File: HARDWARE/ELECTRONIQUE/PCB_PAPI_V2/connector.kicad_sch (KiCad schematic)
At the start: 20 parts, among them J1 USB4110-GF-A, J3 XT30PW-M, J5 SM12B-SRSS-TB_LF__SN_

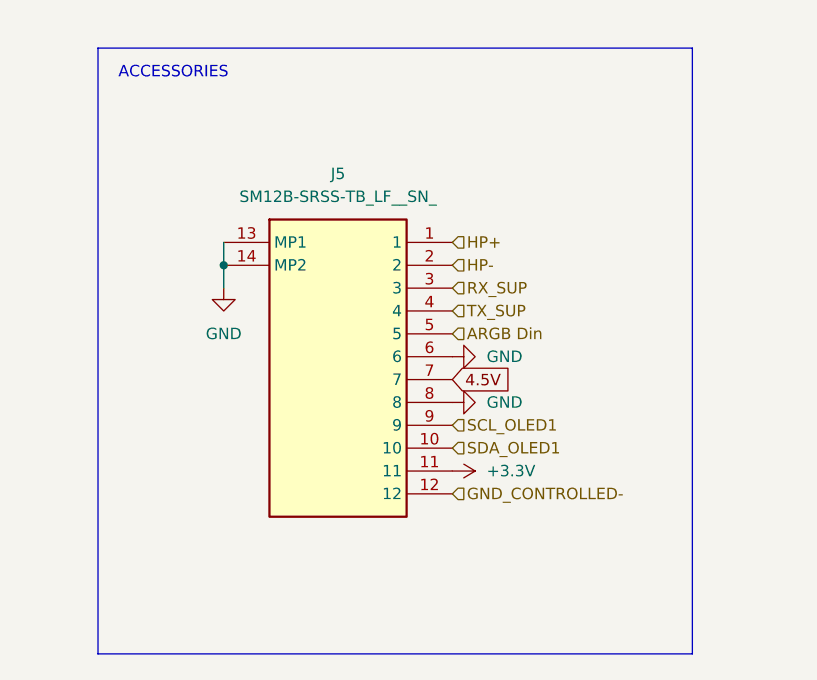
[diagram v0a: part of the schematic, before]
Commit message: up
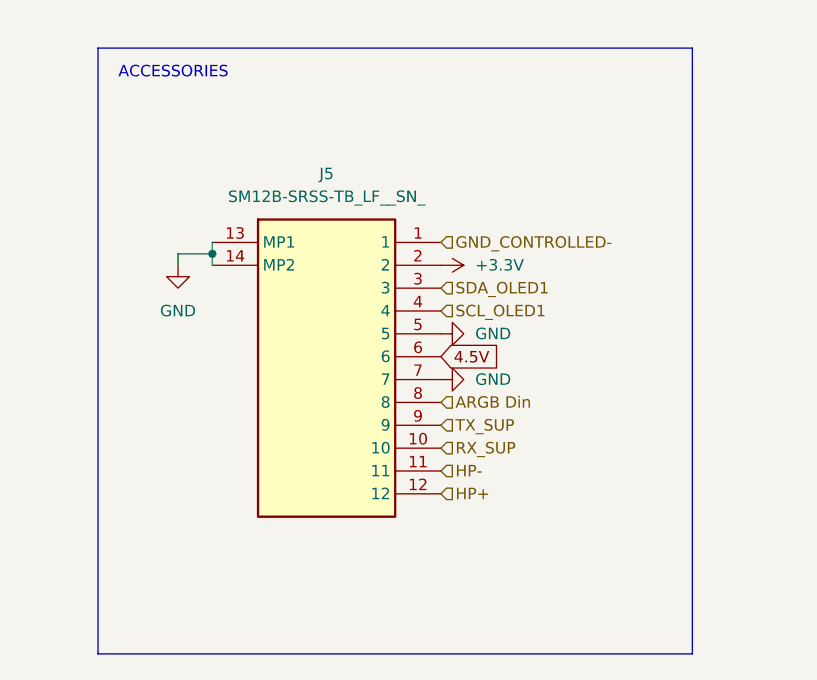
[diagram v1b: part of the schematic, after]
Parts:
- USBJUMP1: footprint Connector_PinHeader_1.00mm:PinHeader_2x04_P1.00mm_Vertical_SMD -> Connector_PinHeader_1.27mm:PinHeader_2x04_P1.27mm_Vertical_SMD
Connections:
- net +3.3V: now also J5.2; no longer J5.11
- net 4.5V: now also J5.6; no longer J5.7
- net ARGB Din: now also J5.8; no longer J5.5
- net GND: now also J5.5, J5.7; no longer J5.6, J5.8
- net GND_CONTROLLED-: now also J5.1; no longer J5.12
- net HP+: now also J5.12; no longer J5.1
- net HP-: now also J5.11; no longer J5.2
- net RX_SUP: now also J5.10; no longer J5.3
- net SCL_OLED1: now also J5.4; no longer J5.9
- net SDA_OLED1: now also J5.3; no longer J5.10
- net TX_SUP: now also J5.9; no longer J5.4
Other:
- moved on the sheet: J5
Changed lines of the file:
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@@
 	)
 	(junction
-		(at 48.26 138.43)
-		(diameter 0)
-		(color 0 0 0 0)
-	)
-	(junction
 		(at 81.28 34.29)
 		(diameter 0)
@@
 	)
 	(junction
+		(at 46.99 137.16)
+		(diameter 0)
+		(color 0 0 0 0)
+	)
+	(junction
 		(at 91.44 60.96)
 		(diameter 0)
@@
 	(wire
 		(pts
-			(xy 48.26 138.43) (xy 48.26 140.97)
+			(xy 43.18 137.16) (xy 43.18 138.43)
 		)
 		(stroke
@@
 	(wire
 		(pts
+			(xy 46.99 137.16) (xy 43.18 137.16)
+		)
+		(stroke
+			(width 0)
+			(type default)
+		)
+	)
+	(wire
+		(pts
 			(xy 358.14 154.94) (xy 358.14 153.67)
 		)
@@
 	(wire
 		(pts
+			(xy 46.99 137.16) (xy 46.99 138.43)
+		)
+		(stroke
+			(width 0)
+			(type default)
+		)
+	)
+	(wire
+		(pts
 			(xy 281.94 215.9) (xy 259.08 215.9)
 		)
@@
 	(wire
 		(pts
-			(xy 48.26 135.89) (xy 48.26 138.43)
+			(xy 91.44 59.69) (xy 91.44 60.96)
 		)
 		(stroke
@@
 	(wire
 		(pts
-			(xy 91.44 59.69) (xy 91.44 60.96)
+			(xy 200.66 50.8) (xy 201.93 50.8)
 		)
 		(stroke
@@
 	(wire
 		(pts
-			(xy 200.66 50.8) (xy 201.93 50.8)
+			(xy 345.44 43.18) (xy 342.9 43.18)
 		)
 		(stroke
@@
 	(wire
 		(pts
-			(xy 345.44 43.18) (xy 342.9 43.18)
+			(xy 68.58 80.01) (xy 74.93 80.01)
 		)
 		(stroke
@@
 	(wire
 		(pts
-			(xy 68.58 80.01) (xy 74.93 80.01)
+			(xy 46.99 135.89) (xy 46.99 137.16)
 		)
 		(stroke
@@
 	(global_label "4.5V"
 		(shape input)
-		(at 73.66 151.13 0)
+		(at 72.39 148.59 0)
 		(fields_autoplaced yes)
 		(effects
@@
 		)
 		(property "Intersheetrefs" "${INTERSHEET_REFS}"
-			(at 80.7576 151.13 0)
+			(at 79.4876 148.59 0)
 			(effects
 				(font
@@
 	(hierarchical_label "RX_SUP"
 		(shape input)
-		(at 73.66 140.97 0)
+		(at 72.39 158.75 0)
 		(effects
 			(font
@@
 	(hierarchical_label "SCL_OLED1"
 		(shape input)
-		(at 73.66 156.21 0)
+		(at 72.39 143.51 0)
 		(effects
 			(font
@@
 	(hierarchical_label "HP+"
 		(shape input)
-		(at 73.66 135.89 0)
+		(at 72.39 163.83 0)
 		(effects
 			(font
@@
 	(hierarchical_label "GND_CONTROLLED-"
 		(shape input)
-		(at 73.66 163.83 0)
+		(at 72.39 135.89 0)
 		(effects
 			(font
@@
 	(hierarchical_label "ARGB Din"
 		(shape input)
-		(at 73.66 146.05 0)
+		(at 72.39 153.67 0)
 		(effects
 			(font
@@
 	(hierarchical_label "SDA_OLED1"
 		(shape input)
-		(at 73.66 158.75 0)
+		(at 72.39 140.97 0)
 		(effects
 			(font
@@
 	(hierarchical_label "HP-"
 		(shape input)
-		(at 73.66 138.43 0)
+		(at 72.39 161.29 0)
 		(effects
 			(font
@@
 	(hierarchical_label "TX_SUP"
 		(shape input)
-		(at 73.66 143.51 0)
+		(at 72.39 156.21 0)
 		(effects
 			(font
@@
 			)
 		)
-		(property "Footprint" "Connector_PinHeader_1.00mm:PinHeader_2x04_P1.00mm_Vertical_SMD"
+		(property "Footprint" "Connector_PinHeader_1.27mm:PinHeader_2x04_P1.27mm_Vertical_SMD"
 			(at 127 45.72 0)
 			(effects
@@
 	(symbol
 		(lib_id "samacsys:SM12B-SRSS-TB_LF__SN_")
-		(at 48.26 135.89 0)
+		(at 46.99 135.89 0)
 		(unit 1)
 		(exclude_from_sim no)
@@
 		(fields_autoplaced yes)
 		(property "Reference" "J5"
-			(at 60.96 128.27 0)
+			(at 59.69 128.27 0)
 			(effects
 				(font
@@
 		)
 		(property "Value" "SM12B-SRSS-TB_LF__SN_"
-			(at 60.96 130.81 0)
+			(at 59.69 130.81 0)
 			(effects
 				(font
@@
 		)
 		(property "Footprint" "samacsys:SM12BSRSSTBLFSN"
-			(at 69.85 230.81 0)
+			(at 68.58 230.81 0)
 			(effects
 				(font
@@
 		)
 		(property "Datasheet" "https://www.jst-mfg.com/product/pdf/eng/eSH.pdf?67c6d96c290cd"
-			(at 69.85 330.81 0)
+			(at 68.58 330.81 0)
 			(effects
 				(font
@@
 		)
 		(property "Description" "Connector Header Surface Mount, Right Angle 12 position 0.039\" (1.00mm)"
-			(at 48.26 135.89 0)
+			(at 46.99 135.89 0)
 			(effects
 				(font
@@
 		)
 		(property "Height" "2.95"
-			(at 69.85 530.81 0)
+			(at 68.58 530.81 0)
 			(effects
 				(font
@@
 		)
 		(property "Manufacturer_Name" "JST (JAPAN SOLDERLESS TERMINALS)"
-			(at 69.85 630.81 0)
+			(at 68.58 630.81 0)
 			(effects
 				(font
@@
 		)
 		(property "Manufacturer_Part_Number" "SM12B-SRSS-TB(LF)(SN)"
-			(at 69.85 730.81 0)
+			(at 68.58 730.81 0)
 			(effects
 				(font
@@
 		)
 		(property "Mouser Part Number" "N/A"
-			(at 69.85 830.81 0)
+			(at 68.58 830.81 0)
 			(effects
 				(font
@@
 		)
 		(property "Mouser Price/Stock" "https://www.mouser.co.uk/ProductDetail/JST-Commercial/SM12B-SRSS-TBLFSN?qs=QpmGXVUTftGbMQGOEOOssg%3D%3D"
-			(at 69.85 930.81 0)
+			(at 68.58 930.81 0)
 			(effects
 				(font
@@
 		)
 		(property "Arrow Part Number" "SM12B-SRSS-TB(LF)(SN)"
-			(at 69.85 1030.81 0)
+			(at 68.58 1030.81 0)
 			(effects
 				(font
@@
 		)
 		(property "Arrow Price/Stock" "https://www.arrow.com/en/products/sm12b-srss-tb-lf-sn/jst-manufacturing?utm_currency=USD&region=europe"
-			(at 69.85 1130.81 0)
+			(at 68.58 1130.81 0)
 			(effects
 				(font
@@
 	(symbol
 		(lib_id "power:GND")
-		(at 73.66 148.59 90)
-		(mirror x)
+		(at 72.39 151.13 90)
 		(unit 1)
 		(exclude_from_sim no)
@@
 		(fields_autoplaced yes)
 		(property "Reference" "#PWR0105"
-			(at 80.01 148.59 0)
+			(at 78.74 151.13 0)
 			(effects
 				(font
@@
 		)
 		(property "Value" "GND"
-			(at 77.47 148.5899 90)
+			(at 76.2 151.1301 90)
 			(effects
 				(font
@@
 		)
 		(property "Footprint" ""
-			(at 73.66 148.59 0)
+			(at 72.39 151.13 0)
 			(effects
 				(font
@@
 		)
 		(property "Datasheet" ""
-			(at 73.66 148.59 0)
+			(at 72.39 151.13 0)
 			(effects
 				(font
@@
 		)
 		(property "Description" "Power symbol creates a global label with name \"GND\" , ground"
-			(at 73.66 148.59 0)
+			(at 72.39 151.13 0)
 			(effects
 				(font
@@
 	(symbol
 		(lib_id "power:+3.3V")
-		(at 73.66 161.29 270)
-		(mirror x)
+		(at 72.39 138.43 270)
 		(unit 1)
 		(exclude_from_sim no)
@@
 		(fields_autoplaced yes)
 		(property "Reference" "#PWR064"
-			(at 69.85 161.29 0)
+			(at 68.58 138.43 0)
 			(effects
 				(font
@@
 		)
 		(property "Value" "+3.3V"
-			(at 77.47 161.2899 90)
+			(at 76.2 138.4301 90)
 			(effects
 				(font
@@
 		)
 		(property "Footprint" ""
-			(at 73.66 161.29 0)
+			(at 72.39 138.43 0)
 			(effects
 				(font
@@
 		)
 		(property "Datasheet" ""
-			(at 73.66 161.29 0)
+			(at 72.39 138.43 0)
 			(effects
 				(font
@@
 		)
 		(property "Description" "Power symbol creates a global label with name \"+3.3V\""
-			(at 73.66 161.29 0)
+			(at 72.39 138.43 0)
 			(effects
 				(font
@@
 	(symbol
 		(lib_id "power:GND")
-		(at 48.26 140.97 0)
+		(at 43.18 138.43 0)
 		(unit 1)
 		(exclude_from_sim no)
@@
 		(fields_autoplaced yes)
 		(property "Reference" "#PWR089"
-			(at 48.26 147.32 0)
+			(at 43.18 144.78 0)
 			(effects
 				(font
@@
 		)
 		(property "Value" "GND"
-			(at 48.26 146.05 0)
+			(at 43.18 143.51 0)
 			(effects
 				(font
@@
 		)
 		(property "Footprint" ""
-			(at 48.26 140.97 0)
+			(at 43.18 138.43 0)
 			(effects
 				(font
@@
 		)
 		(property "Datasheet" ""
-			(at 48.26 140.97 0)
+			(at 43.18 138.43 0)
 			(effects
 				(font
@@
 		)
 		(property "Description" "Power symbol creates a global label with name \"GND\" , ground"
-			(at 48.26 140.97 0)
+			(at 43.18 138.43 0)
 			(effects
 				(font
@@
 	(symbol
 		(lib_id "power:GND")
-		(at 73.66 153.67 90)
-		(mirror x)
+		(at 72.39 146.05 90)
 		(unit 1)
 		(exclude_from_sim no)
@@
 		(fields_autoplaced yes)
 		(property "Reference" "#PWR082"
-			(at 80.01 153.67 0)
+			(at 78.74 146.05 0)
 			(effects
 				(font
@@
 		)
 		(property "Value" "GND"
-			(at 77.47 153.6699 90)
+			(at 76.2 146.0501 90)
 			(effects
 				(font
@@
 		)
 		(property "Footprint" ""
-			(at 73.66 153.67 0)
+			(at 72.39 146.05 0)
 			(effects
 				(font
@@
 		)
 		(property "Datasheet" ""
-			(at 73.66 153.67 0)
+			(at 72.39 146.05 0)
 			(effects
 				(font
@@
 		)
 		(property "Description" "Power symbol creates a global label with name \"GND\" , ground"
-			(at 73.66 153.67 0)
+			(at 72.39 146.05 0)
 			(effects
 				(font
